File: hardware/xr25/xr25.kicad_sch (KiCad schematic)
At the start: 1 part, among them J3 XR25_INTERFACE

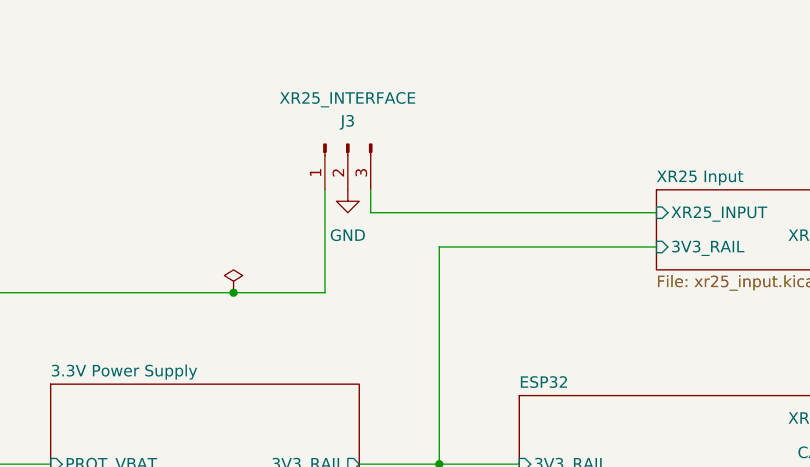
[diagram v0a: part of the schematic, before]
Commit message: finished first version of pcb
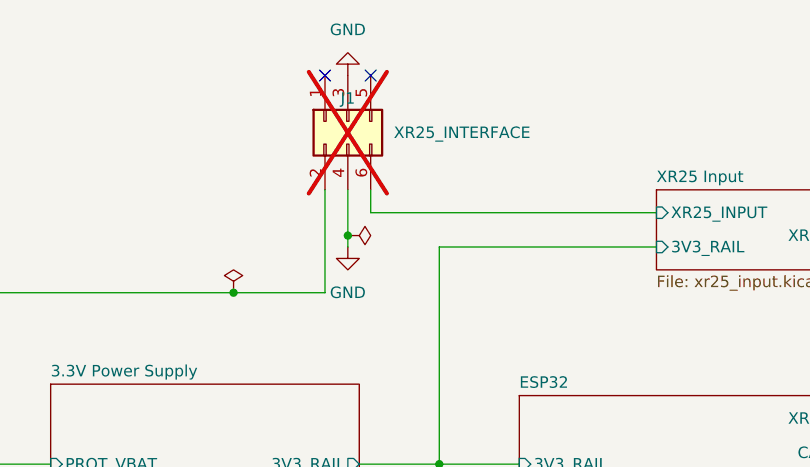
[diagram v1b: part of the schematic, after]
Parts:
- J1: renamed from J3; footprint (none) -> Connector_PinHeader_2.54mm:PinHeader_2x03_P2.54mm_Vertical; symbol Connector:Conn_01x03_Pin -> Connector_Generic:Conn_02x03_Odd_Even; now not fitted
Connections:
- net GND: now also J1.3 (Pin_3), J1.4 (Pin_4); no longer J1.2 (Pin_2)
- net Protection Circuit/VBAT: now also J1.2 (Pin_2); no longer J1.1 (Pin_1)
- net XR25 Input/XR25_INPUT: now also J1.6 (Pin_6); no longer J1.3 (Pin_3)
- no-connect marks 0 -> 2
